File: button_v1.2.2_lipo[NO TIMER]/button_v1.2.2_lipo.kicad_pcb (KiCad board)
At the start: 2 copper layers, 21 x 41.7 mm, 17 parts, among them J1 Conn_01x05_Female, SW1 SW_Push, SW2 SW_Push, U2 AP2112K-3.3, X1 ESP-12E

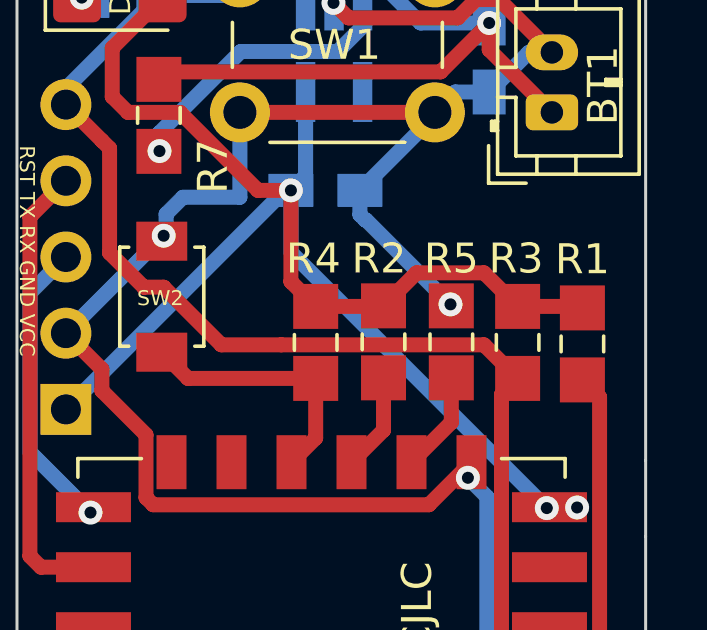
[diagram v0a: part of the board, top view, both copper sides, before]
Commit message: :rocket:  :new_moon:
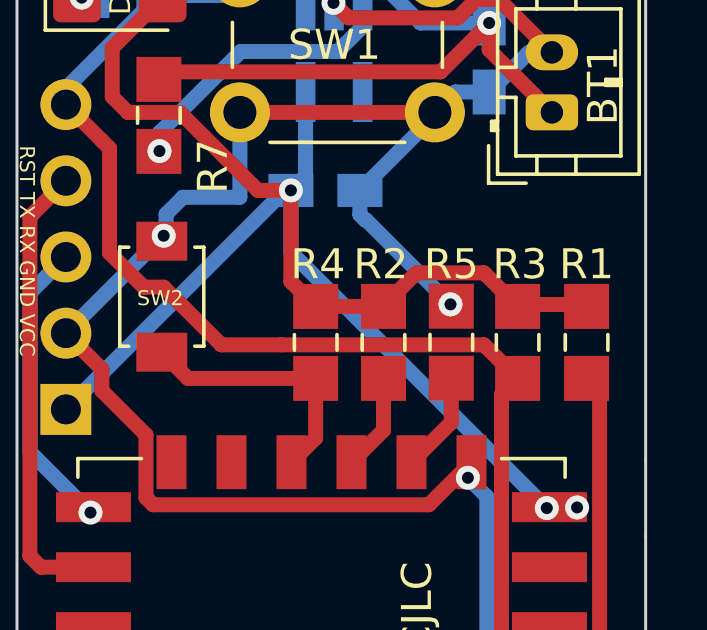
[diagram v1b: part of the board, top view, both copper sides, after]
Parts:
- moved R1 0.15 mm to (134.6, 74.2)

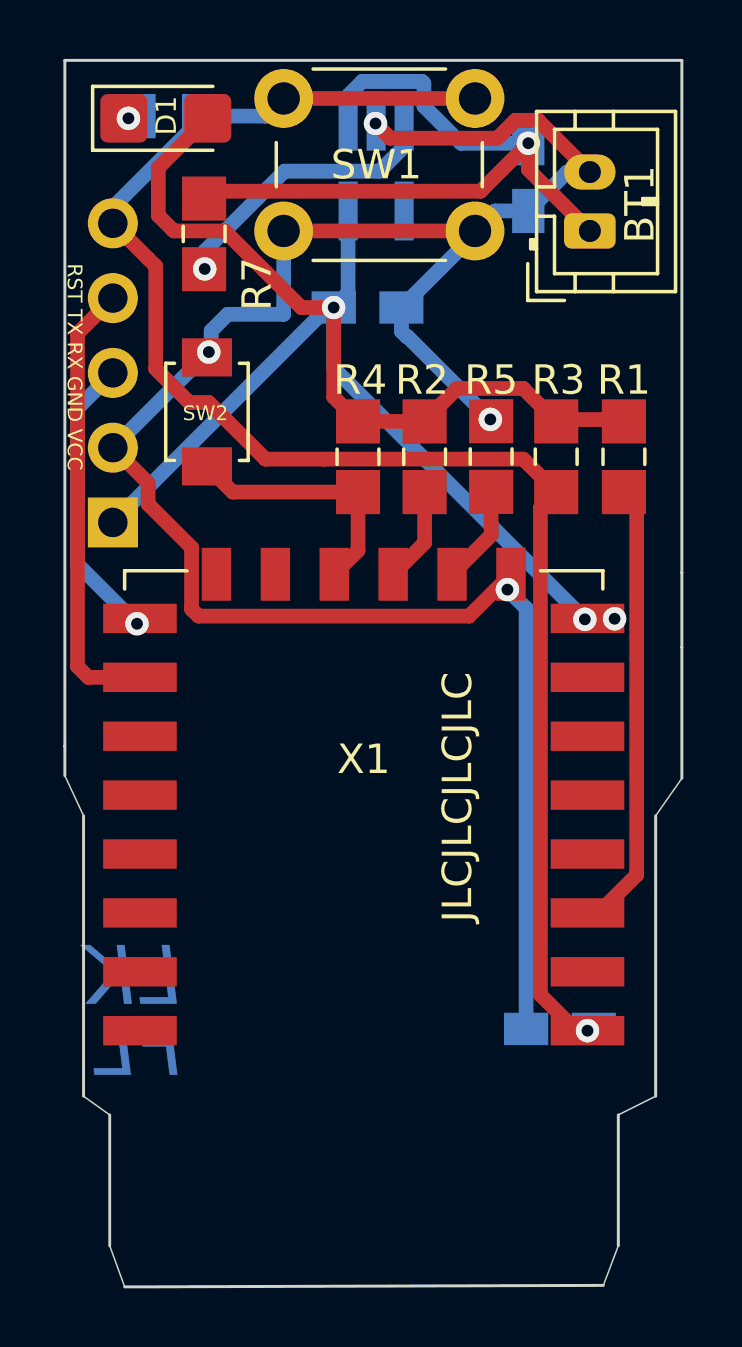
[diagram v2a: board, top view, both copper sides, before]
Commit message: Silkscreen Update
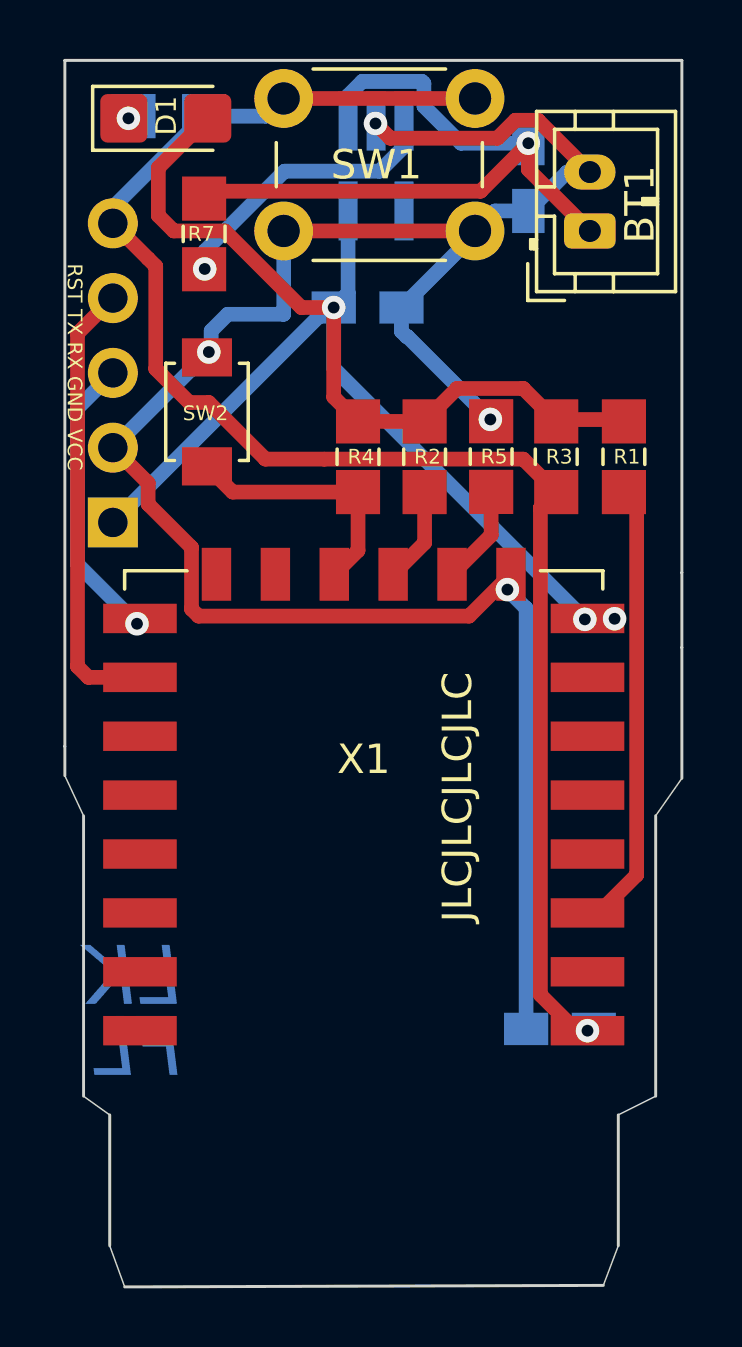
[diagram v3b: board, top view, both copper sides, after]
